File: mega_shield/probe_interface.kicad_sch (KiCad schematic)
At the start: 11 parts, among them J22 T4041017031-000, U27 4N35

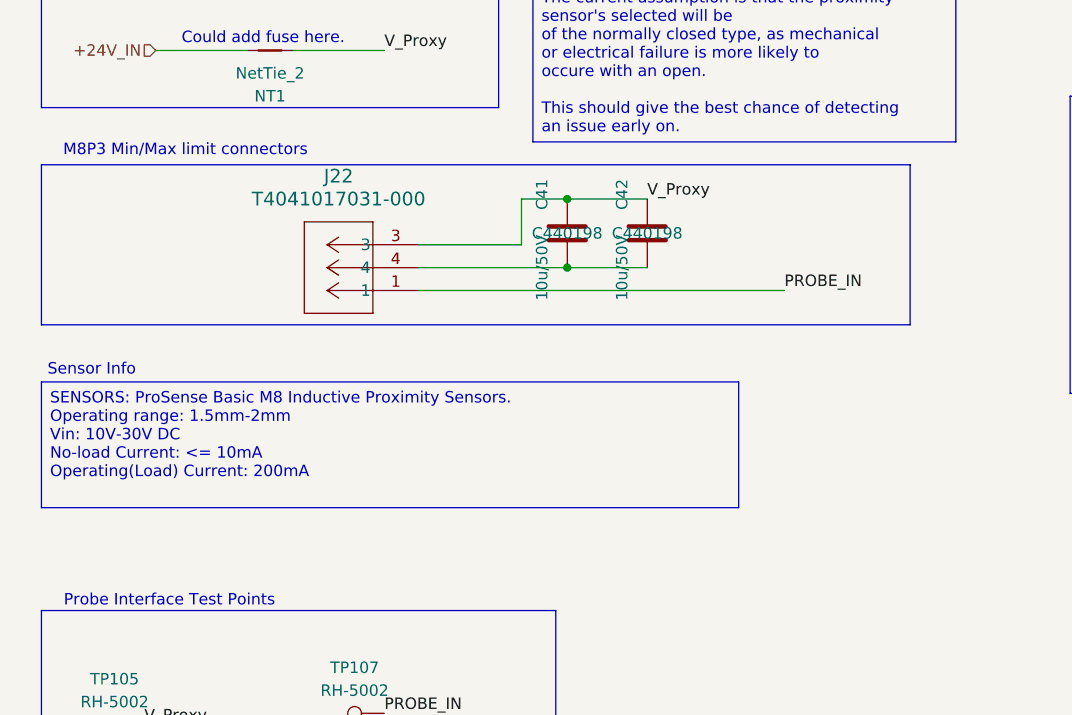
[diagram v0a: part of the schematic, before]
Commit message: mega_shield, marked circular components as DNP, added jlcpcb numbers to 90degree terminal blocks.
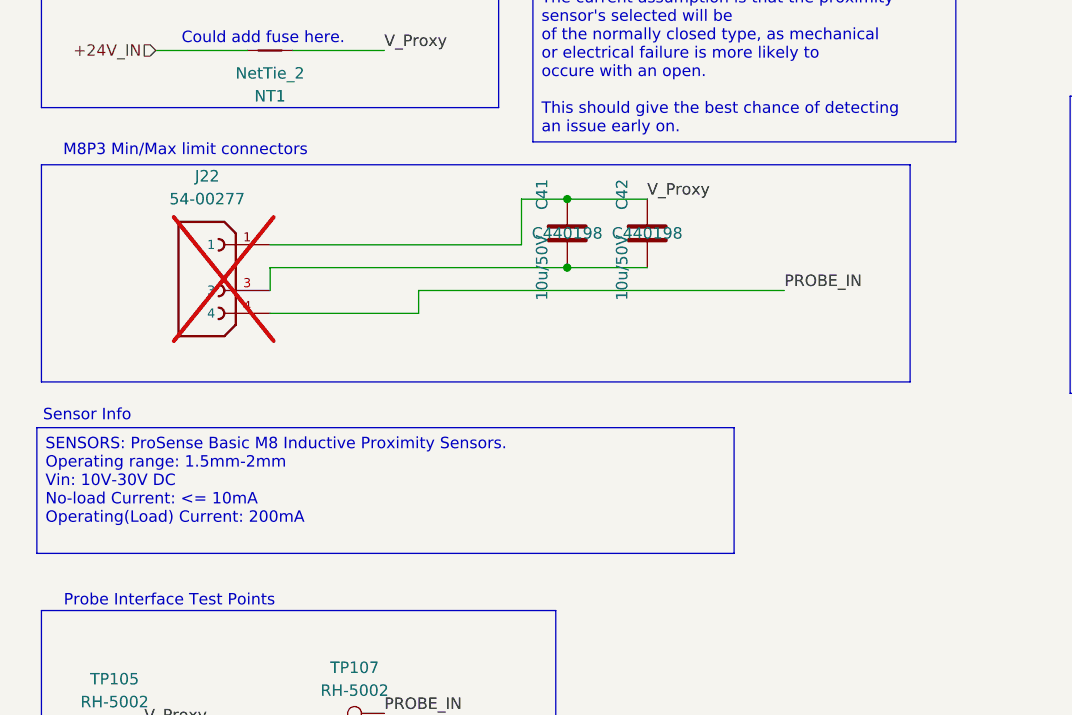
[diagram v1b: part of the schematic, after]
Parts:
- removed J22: T4041017031-000, footprints:CONN_T4041017031-000_TEC, symbol mega_shield:T4041017031-000
- added J22: 54-00277, footprints:TENSILITY_54-00277, symbol 54-00277:54-00277
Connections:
- net PROBE_IN: now also J22.4
- net V_Proxy: now also J22.1
- net at C41.2, C42.2: now also J22.3
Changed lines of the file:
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@@
 	(rectangle
 		(start 25.4 45.72)
-		(end 121.92 63.5)
+		(end 121.92 69.85)
 		(stroke
 			(width 0)
@@
 	(text "Sensor Info"
 		(exclude_from_sim no)
-		(at 30.988 68.58 0)
+		(at 30.48 73.66 0)
 		(effects
 			(font
@@
 	(text_box "SENSORS: ProSense Basic M8 Inductive Proximity Sensors.\nOperating range: 1.5mm-2mm\nVin: 10V-30V DC\nNo-load Current: <= 10mA\nOperating(Load) Current: 200mA\n"
 		(exclude_from_sim no)
-		(at 25.4 69.85 0)
+		(at 24.892 74.93 0)
 		(size 77.47 13.97)
 		(margins 0.9525 0.9525 0.9525 0.9525)
@@
 	(wire
 		(pts
-			(xy 83.82 57.15) (xy 67.31 57.15)
-		)
-		(stroke
-			(width 0)
-			(type default)
-		)
-	)
-	(wire
-		(pts
-			(xy 67.31 54.61) (xy 78.74 54.61)
-		)
-		(stroke
-			(width 0)
-			(type default)
-		)
-	)
-	(wire
-		(pts
 			(xy 92.71 57.15) (xy 83.82 57.15)
 		)
@@
 	(wire
 		(pts
+			(xy 50.8 57.15) (xy 50.8 59.69)
+		)
+		(stroke
+			(width 0)
+			(type default)
+		)
+	)
+	(wire
+		(pts
 			(xy 187.96 57.15) (xy 194.31 57.15)
 		)
@@
 	(wire
 		(pts
+			(xy 50.8 54.61) (xy 78.74 54.61)
+		)
+		(stroke
+			(width 0)
+			(type default)
+		)
+	)
+	(wire
+		(pts
 			(xy 182.88 63.5) (xy 182.88 59.69)
 		)
@@
 	(wire
 		(pts
+			(xy 50.8 57.15) (xy 83.82 57.15)
+		)
+		(stroke
+			(width 0)
+			(type default)
+		)
+	)
+	(wire
+		(pts
 			(xy 107.95 59.69) (xy 67.31 59.69)
 		)
@@
 	(wire
 		(pts
+			(xy 50.8 62.23) (xy 67.31 62.23)
+		)
+		(stroke
+			(width 0)
+			(type default)
+		)
+	)
+	(wire
+		(pts
 			(xy 78.74 54.61) (xy 78.74 49.53)
 		)
@@
 		(pts
 			(xy 182.88 59.69) (xy 181.61 59.69)
+		)
+		(stroke
+			(width 0)
+			(type default)
+		)
+	)
+	(wire
+		(pts
+			(xy 67.31 59.69) (xy 67.31 62.23)
 		)
 		(stroke
@@
 	)
 	(symbol
-		(lib_id "mega_shield:T4041017031-000")
-		(at 67.31 59.69 180)
-		(unit 1)
-		(exclude_from_sim no)
-		(in_bom yes)
-		(on_board yes)
-		(dnp no)
-		(fields_autoplaced yes)
-		(property "Reference" "J22"
-			(at 58.42 46.99 0)
-			(effects
-				(font
-					(size 1.524 1.524)
-				)
-			)
-		)
-		(property "Value" "T4041017031-000"
-			(at 58.42 49.53 0)
-			(effects
-				(font
-					(size 1.524 1.524)
-				)
-			)
-		)
-		(property "Footprint" "footprints:CONN_T4041017031-000_TEC"
-			(at 67.31 59.69 0)
-			(effects
-				(font
-					(size 1.27 1.27)
-					(italic yes)
-				)
-				(hide yes)
-			)
-		)
-		(property "Datasheet" "https://www.te.com/commerce/DocumentDelivery/DDEController?Action=srchrtrv&DocNm=1-1773701-8_M8M12_CONNECTOR_SYSTEM&DocType=Catalog+Section&DocLang=English&PartCntxt=1838895-1&DocFormat=pdf"
-			(at 67.31 59.69 0)
-			(effects
-				(font
-					(size 1.27 1.27)
-					(italic yes)
-				)
-				(hide yes)
-			)
-		)
-		(property "Description" ""
-			(at 67.31 59.69 0)
-			(effects
-				(font
-					(size 1.27 1.27)
-				)
-				(hide yes)
-			)
-		)
-		(pin "4"
-		)
-		(pin "1"
-		)
-		(pin "3"
-		)
-		(instances
-			(project ""
-				(path "/554fcf27-dc63-4666-abbc-7481d15942c4/e56aebf0-16bd-4ef0-8607-05648fa38946"
-					(reference "J22")
-					(unit 1)
-				)
-			)
-		)
-	)
-	(symbol
 		(lib_id "power:GND")
 		(at 165.1 63.5 0)
@@
 					(unit 1)
 				)
+			)
+		)
+	)
+	(symbol
+		(lib_id "54-00277:54-00277")
+		(at 43.18 57.15 0)
+		(unit 1)
+		(exclude_from_sim no)
+		(in_bom yes)
+		(on_board yes)
+		(dnp yes)
+		(fields_autoplaced yes)
+		(property "Reference" "J22"
+			(at 43.815 46.99 0)
+			(effects
+				(font
+					(size 1.27 1.27)
+				)
+			)
+		)
+		(property "Value" "54-00277"
+			(at 43.815 49.53 0)
+			(effects
+				(font
+					(size 1.27 1.27)
+				)
+			)
+		)
+		(property "Footprint" "footprints:TENSILITY_54-00277"
+			(at 43.18 57.15 0)
+			(effects
+				(font
+					(size 1.27 1.27)
+				)
+				(justify bottom)
+				(hide yes)
+			)
+		)
+		(property "Datasheet" ""
+			(at 43.18 57.15 0)
+			(effects
+				(font
+					(size 1.27 1.27)
+				)
+				(hide yes)
+			)
+		)
+		(property "Description" ""
+			(at 43.18 57.15 0)
+			(effects
+				(font
+					(size 1.27 1.27)
+				)
+				(hide yes)
+			)
+		)
+		(property "MF" "Tensility International Corp"
+			(at 43.18 57.15 0)
+			(effects
+				(font
+					(size 1.27 1.27)
+				)
+				(justify bottom)
+				(hide yes)
+			)
+		)
+		(property "MAXIMUM_PACKAGE_HEIGHT" "20.2 mm"
+			(at 43.18 57.15 0)
+			(effects
+				(font
+					(size 1.27 1.27)
+				)
+				(justify bottom)
+				(hide yes)
+			)
+		)
+		(property "Package" "None"
+			(at 43.18 57.15 0)
+			(effects
+				(font
+					(size 1.27 1.27)
+				)
+				(justify bottom)
+				(hide yes)
+			)
+		)
+		(property "Price" "None"
+			(at 43.18 57.15 0)
+			(effects
+				(font
+					(size 1.27 1.27)
+				)
+				(justify bottom)
+				(hide yes)
+			)
+		)
+		(property "Check_prices" "https://www.snapeda.com/parts/54-00277/Tensility/view-part/?ref=eda"
+			(at 43.18 57.15 0)
+			(effects
+				(font
+					(size 1.27 1.27)
+				)
+				(justify bottom)
+				(hide yes)
+			)
+		)
+		(property "STANDARD" "Manufacturer Recommendations"
+			(at 43.18 57.15 0)
+			(effects
+				(font
+					(size 1.27 1.27)
+				)
+				(justify bottom)
+				(hide yes)
+			)
+		)
+		(property "PARTREV" "A"
+			(at 43.18 57.15 0)
+			(effects
+				(font
+					(size 1.27 1.27)
+				)
+				(justify bottom)
+				(hide yes)
+			)
+		)
+		(property "SnapEDA_Link" "https://www.snapeda.com/parts/54-00277/Tensility/view-part/?ref=snap"
+			(at 43.18 57.15 0)
+			(effects
+				(font
+					(size 1.27 1.27)
+				)
+				(justify bottom)
+				(hide yes)
+			)
+		)
+		(property "MP" "54-00277"
+			(at 43.18 57.15 0)
+			(effects
+				(font
+					(size 1.27 1.27)
+				)
+				(justify bottom)
+				(hide yes)
+			)
+		)
+		(property "Description_1" "Connector, 3 pin M8 A-code socket, 8x22.4 mm, gold plated, panel mount, PCB, IP67"
+			(at 43.18 57.15 0)
+			(effects
+				(font
+					(size 1.27 1.27)
+				)
+				(justify bottom)
+				(hide yes)
+			)
+		)
+		(property "Availability" "In Stock"
+			(at 43.18 57.15 0)
+			(effects
+				(font
+					(size 1.27 1.27)
+				)
+				(justify bottom)
+				(hide yes)
+			)
+		)
+		(property "MANUFACTURER" "Tensility"
+			(at 43.18 57.15 0)
+			(effects
+				(font
+					(size 1.27 1.27)
+				)
+				(justify bottom)
+				(hide yes)
+			)
+		)
+		(pin "1"
+		)
+		(pin "3"
+		)
+		(pin "4"
+		)
+		(instances
+			(project ""
+				(path "/554fcf27-dc63-4666-abbc-7481d15942c4/e56aebf0-16bd-4ef0-8607-05648fa38946"
+					(reference "J22")
+					(unit 1)
+				)
